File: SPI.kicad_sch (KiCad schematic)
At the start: 11 parts, among them IC3 SRAM, J4 SD_Card, J5 SPI2, J6 SPI1, U2 EEPROM

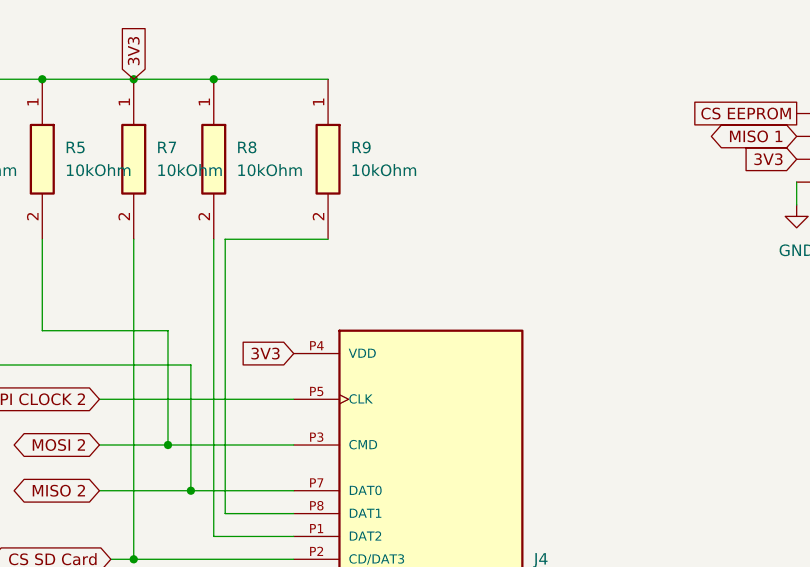
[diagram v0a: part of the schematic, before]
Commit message: initial PCB draft!
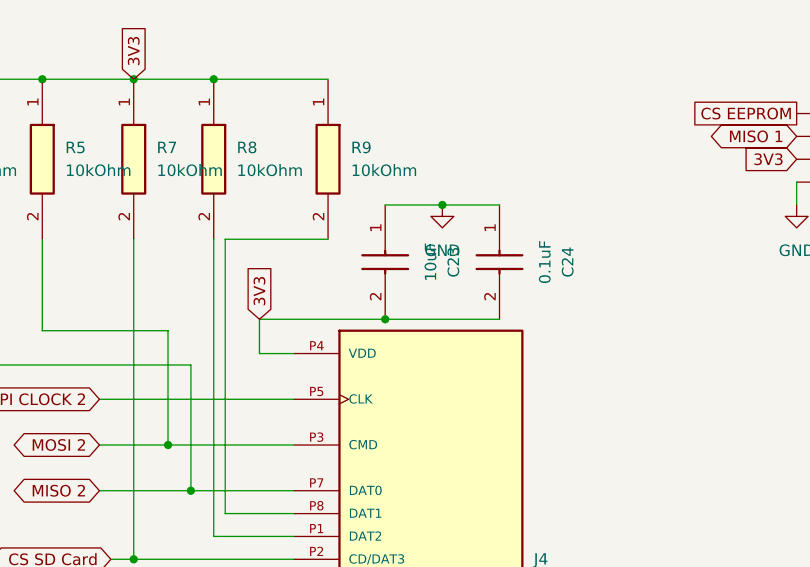
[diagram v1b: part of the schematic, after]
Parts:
- added C23: 10uF, Capacitor_SMD:C_0805_2012Metric, symbol group127:0805Capacitor
- added C24: 0.1uF, Capacitor_SMD:C_0805_2012Metric, symbol group127:0805Capacitor
- IC3: footprint (none) -> group127:SRAM
- J4: footprint (none) -> group127:SDCard
- U2: footprint (none) -> group127:EEPROM
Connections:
- net 3V3: now also C23.2, C24.2
- net GND: now also C23.1, C24.1
